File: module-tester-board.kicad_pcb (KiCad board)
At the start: 2 copper layers, 101.6 x 53.3 mm, 26 parts, among them J1 Conn_01x08_Male, J2 Barrel_Jack, J4 Tester Points, SW1 SW_DIP_x04, U1 LT8330, U4 MCP2515-EST, U5 ATA6560,1, Y1 20MHz

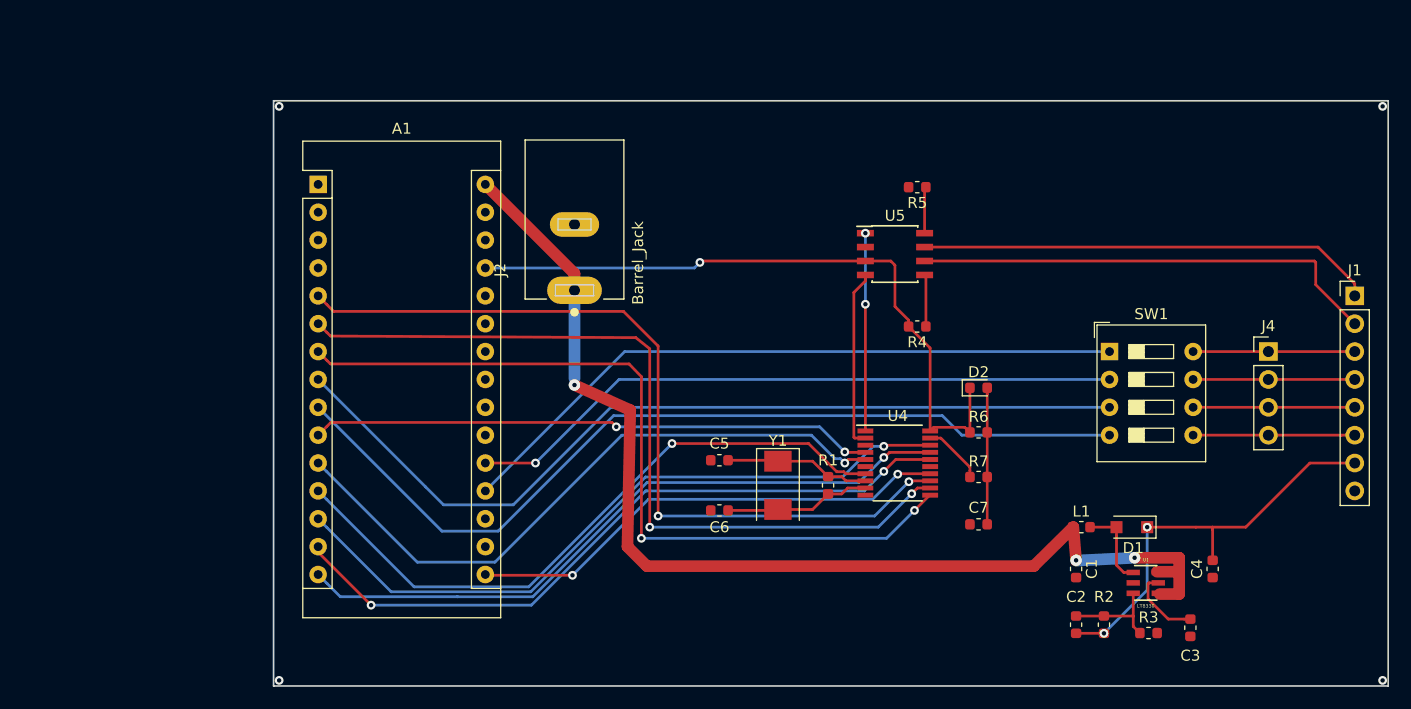
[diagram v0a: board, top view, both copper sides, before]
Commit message: 0.0.11 First version of traces
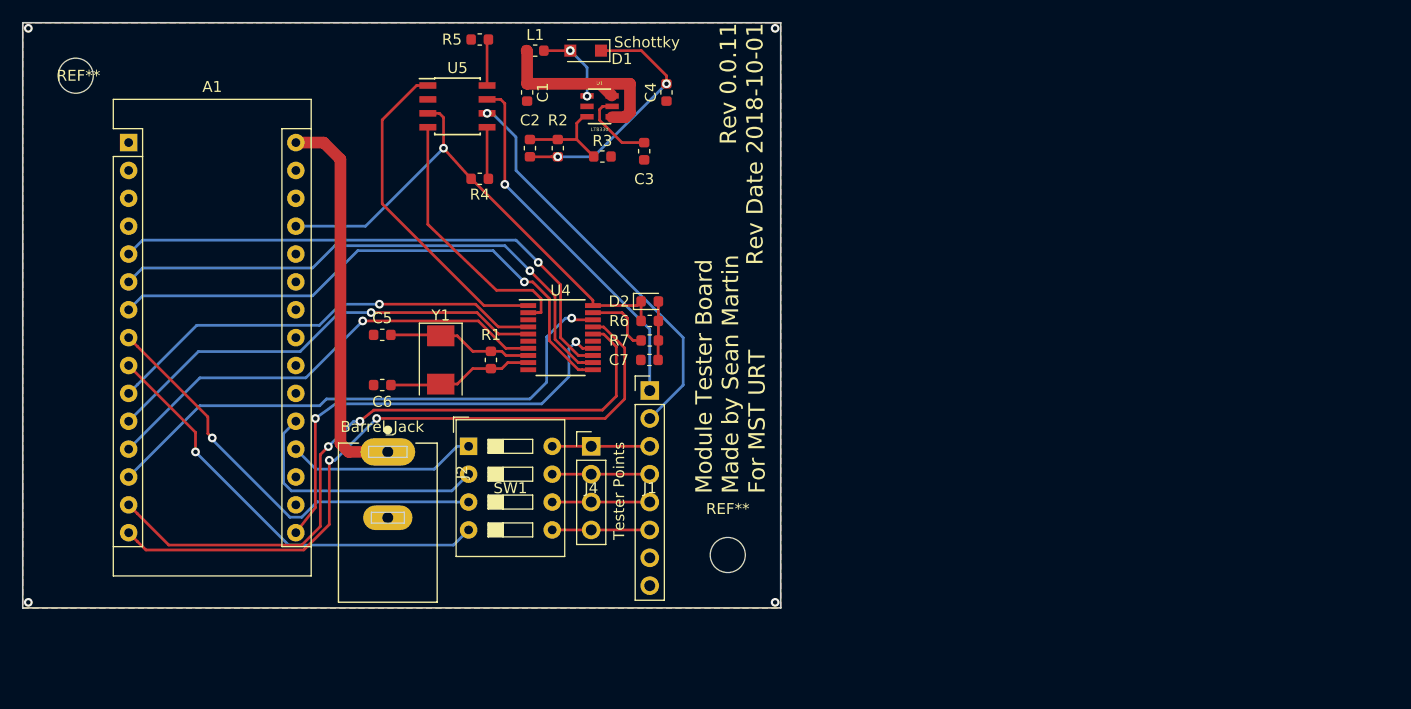
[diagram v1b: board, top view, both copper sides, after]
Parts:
- added REF**: , MountingHole:MountingHole_3.2mm_M3, F.Cu at (123.2, 71.4)
- added REF**: , MountingHole:MountingHole_3.2mm_M3, F.Cu at (182.6, 115.1)
- D1: value D_Schottky -> Schottky
- J1: value Conn_01x08_Male -> (none)
- SW1: value SW_DIP_x04 -> (none)
- U4: value MCP2515-EST -> MCP2515
- moved C1 66.3 mm to (164.3, 72.9)
- moved C2 66.1 mm to (164.6, 78.0)
- moved C3 66.1 mm to (175.0, 78.3)
- moved C4 66.1 mm to (177.0, 72.9)
- moved D1 66.1 mm to (169.7, 69.1)
- moved L1 66.1 mm to (165.1, 69.1)
- moved R2 66.1 mm to (167.1, 78.0)
- moved R3 66.1 mm to (171.2, 78.7)
- moved U1 66.1 mm to (170.9, 74.2)
- moved J1 64.8 mm to (175.5, 100.1)
- moved J4 62.3 mm to (170.2, 105.2)
- moved SW1 59.1 mm to (159.0, 105.2)
- moved U5 42.1 mm to (158.0, 74.2)
- moved R4 42.1 mm to (160.0, 80.8)
- moved R5 42.1 mm to (160.0, 68.1)
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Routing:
- net +12V: track 103.5 -> 54.1 mm, vias 3 -> 0
- net A0: track 62.2 -> 17.4 mm
- net PWM1: track 81.9 -> 39.4 mm, vias 0 -> 1
- net PWM0: track 80.6 -> 39.3 mm, vias 0 -> 1
- net A1: track 60.1 -> 23.9 mm, vias 1 -> 0
- net INT: track 74.5 -> 50.0 mm, vias 2 -> 1
- net RX0: track 74.3 -> 50.6 mm, vias 2 -> 1
- net RX1: track 73.1 -> 51.3 mm, vias 2 -> 1
- net TX1: track 59.6 -> 41.3 mm
- net TX2: track 60.1 -> 42.3 mm
- net +48V: track 38.2 -> 22.9 mm
- net +5V: track 62.2 -> 47.5 mm
- net SS: track 64.1 -> 50.8 mm
- net Net-(U4-Pad1): track 18.2 -> 30.3 mm, vias 2 -> 0
- net TX0: track 51.5 -> 40.6 mm, vias 2 -> 1
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- added copper zone on B.Cu, net GND
- added copper zone on F.Cu, net GND
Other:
- board size 101.6 x 53.3 mm -> 69.1 x 53.3 mm
- board text added: "Module Tester Board Made by Sean Martin For MST URT"
- board text added: "Rev 0.0.11 Rev Date 2018-10-01"
